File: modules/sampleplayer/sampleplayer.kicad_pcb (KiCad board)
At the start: 2 copper layers, 3 parts, among them J1 AudioJack2_SwitchT, U1 ESP32-DEVKIT-V1

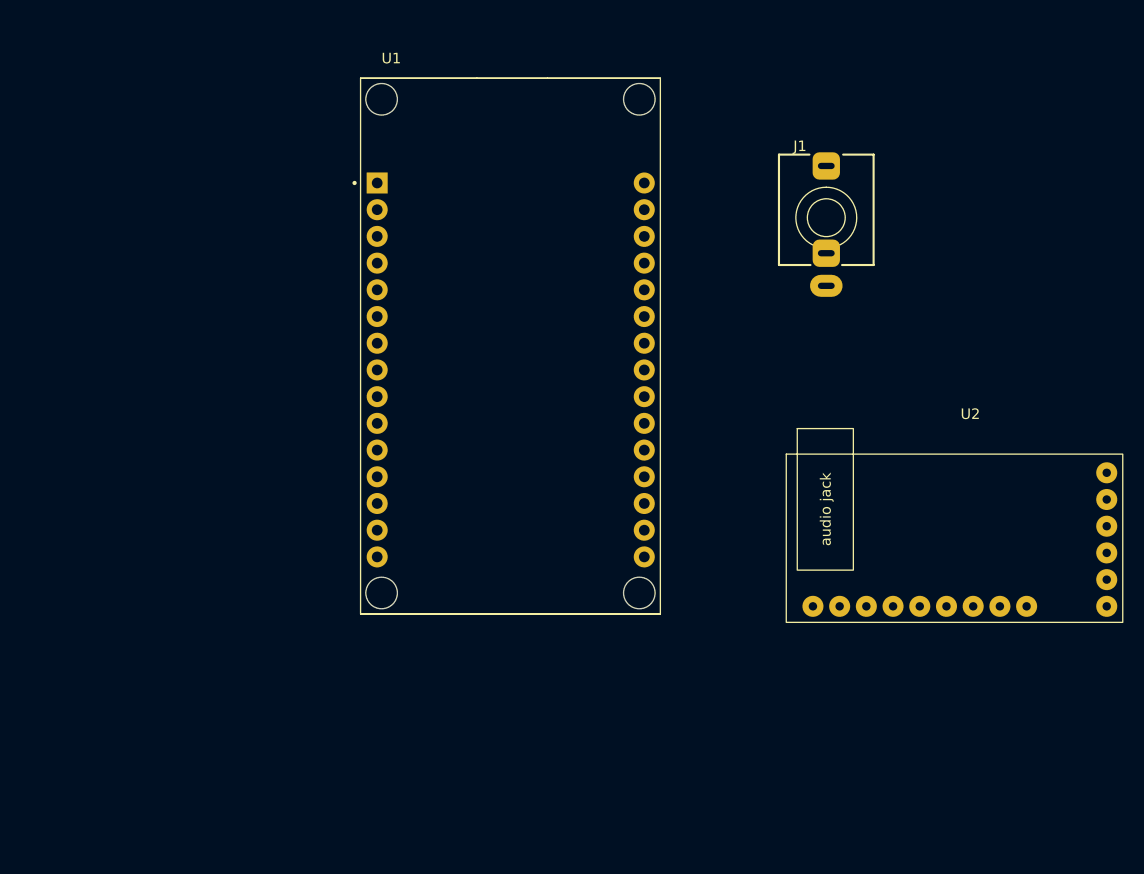
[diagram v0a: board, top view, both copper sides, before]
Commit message: sampleplayer update
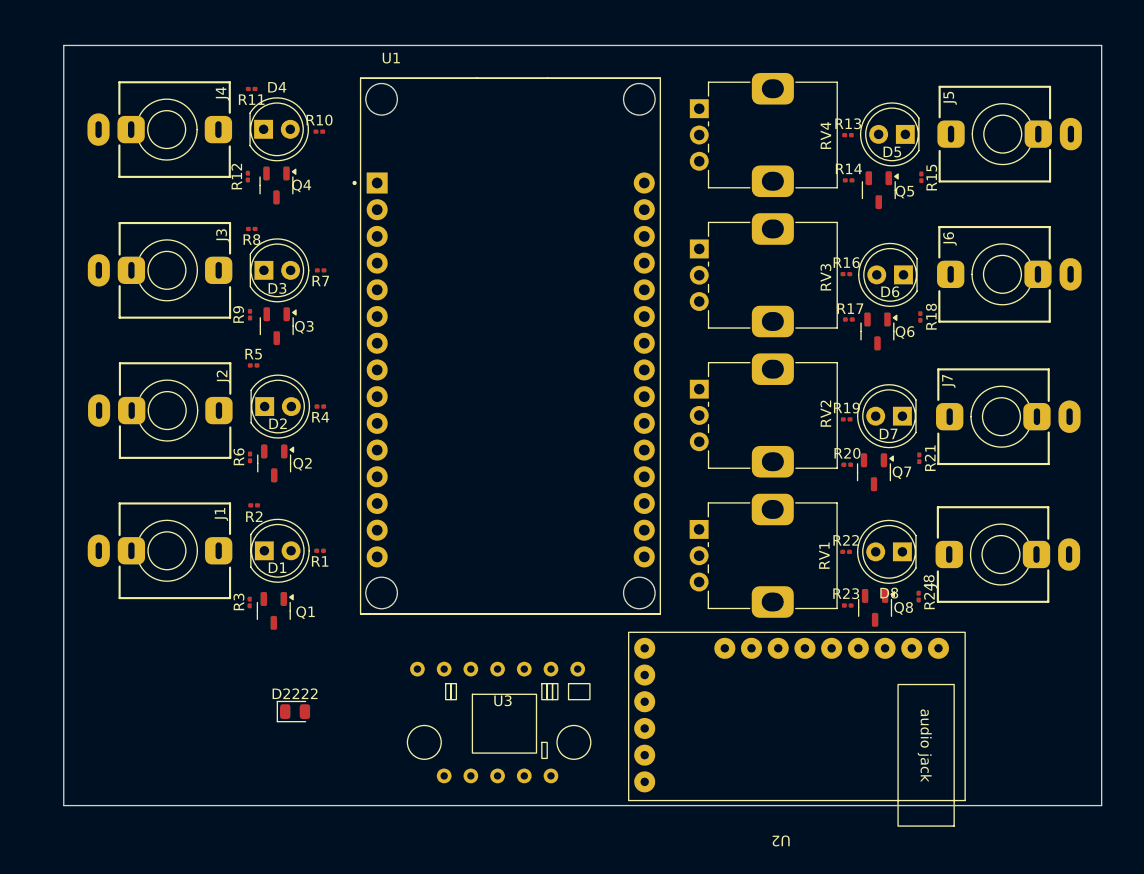
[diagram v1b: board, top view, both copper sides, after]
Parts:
- added D1: 5mm LED, LED_THT:LED_D5.0mm, F.Cu at (124.4, 123.0)
- added D2: 5mm LED, LED_THT:LED_D5.0mm, F.Cu at (124.4, 109.3)
- added D2222: KT-0805G, LED_SMD:LED_0805_2012Metric, F.Cu at (127.3, 138.3)
- added D3: 5mm LED, LED_THT:LED_D5.0mm, F.Cu at (124.3, 96.3)
- added D4: 5mm LED, LED_THT:LED_D5.0mm, F.Cu at (124.3, 82.9)
- added D5: 5mm LED, LED_THT:LED_D5.0mm, F.Cu at (185.3, 83.4)
- added D6: 5mm LED, LED_THT:LED_D5.0mm, F.Cu at (185.1, 96.7)
- added D7: 5mm LED, LED_THT:LED_D5.0mm, F.Cu at (185.0, 110.2)
- added D8: 5mm LED, LED_THT:LED_D5.0mm, F.Cu at (185.0, 123.1)
- added J1: trig1, AudioJacks:Jack_3.5mm_QingPu_WQP-PJ301M-12_Vertical, F.Cu at (115.1, 123.0)
- added J2: trig2, AudioJacks:Jack_3.5mm_QingPu_WQP-PJ301M-12_Vertical, F.Cu at (115.1, 109.7)
- added J3: trig3, AudioJacks:Jack_3.5mm_QingPu_WQP-PJ301M-12_Vertical, F.Cu at (115.1, 96.3)
- added J5: trig5, AudioJacks:Jack_3.5mm_QingPu_WQP-PJ301M-12_Vertical, F.Cu at (194.6, 83.4)
- added J6: trig6, AudioJacks:Jack_3.5mm_QingPu_WQP-PJ301M-12_Vertical, F.Cu at (194.6, 96.7)
- added J7: trig7, AudioJacks:Jack_3.5mm_QingPu_WQP-PJ301M-12_Vertical, F.Cu at (194.5, 110.2)
- added J8: trig8, AudioJacks:Jack_3.5mm_QingPu_WQP-PJ301M-12_Vertical, F.Cu at (194.4, 123.3)
- added Q1: SS8050, Package_TO_SOT_SMD:SOT-23-3, F.Cu at (125.3, 128.7)
- added Q2: SS8050, Package_TO_SOT_SMD:SOT-23-3, F.Cu at (125.3, 114.7)
- added Q3: SS8050, Package_TO_SOT_SMD:SOT-23-3, F.Cu at (125.5, 101.6)
- added Q4: SS8050, Package_TO_SOT_SMD:SOT-23-3, F.Cu at (125.5, 88.2)
- added Q5: SS8050, Package_TO_SOT_SMD:SOT-23-3, F.Cu at (182.8, 88.7)
- added Q6: SS8050, Package_TO_SOT_SMD:SOT-23-3, F.Cu at (182.7, 102.1)
- added Q7: SS8050, Package_TO_SOT_SMD:SOT-23-3, F.Cu at (182.3, 115.5)
- added Q8: SS8050, Package_TO_SOT_SMD:SOT-23-3, F.Cu at (182.4, 128.4)
- added R1: 56, Resistor_SMD:R_0201_0603Metric, F.Cu at (129.7, 123.0)
- added R10: 56, Resistor_SMD:R_0201_0603Metric, F.Cu at (129.6, 83.1)
- added R11: 330, Resistor_SMD:R_0201_0603Metric, F.Cu at (123.1, 79.1)
- added R12: 120K, Resistor_SMD:R_0201_0603Metric, F.Cu at (122.8, 87.4)
- added R13: 56, Resistor_SMD:R_0201_0603Metric, F.Cu at (179.9, 83.5)
- added R14: 330, Resistor_SMD:R_0201_0603Metric, F.Cu at (179.9, 87.8)
- added R15: 120K, Resistor_SMD:R_0201_0603Metric, F.Cu at (186.8, 87.5)
- added R16: 56, Resistor_SMD:R_0201_0603Metric, F.Cu at (179.7, 96.7)
- added R17: 330, Resistor_SMD:R_0201_0603Metric, F.Cu at (179.9, 101.0)
- added R18: 120K, Resistor_SMD:R_0201_0603Metric, F.Cu at (186.7, 100.7)
- added R19: 56, Resistor_SMD:R_0201_0603Metric, F.Cu at (179.7, 110.5)
- added R2: 330, Resistor_SMD:R_0201_0603Metric, F.Cu at (123.4, 118.7)
- added R20: 330, Resistor_SMD:R_0201_0603Metric, F.Cu at (179.8, 114.8)
- added R21: 120K, Resistor_SMD:R_0201_0603Metric, F.Cu at (186.6, 114.2)
- added R22: 56, Resistor_SMD:R_0201_0603Metric, F.Cu at (179.7, 123.1)
- added R23: 330, Resistor_SMD:R_0201_0603Metric, F.Cu at (179.8, 128.2)
- added R24: 120K, Resistor_SMD:R_0201_0603Metric, F.Cu at (186.6, 127.3)
- added R3: 120K, Resistor_SMD:R_0201_0603Metric, F.Cu at (123.0, 127.9)
- added R4: 56, Resistor_SMD:R_0201_0603Metric, F.Cu at (129.7, 109.3)
- added R5: 330, Resistor_SMD:R_0201_0603Metric, F.Cu at (123.3, 105.4)
- added R6: 120K, Resistor_SMD:R_0201_0603Metric, F.Cu at (123.0, 114.1)
- added R7: 56, Resistor_SMD:R_0201_0603Metric, F.Cu at (129.7, 96.3)
- added R8: 330, Resistor_SMD:R_0201_0603Metric, F.Cu at (123.2, 92.4)
- added R9: 120K, Resistor_SMD:R_0201_0603Metric, F.Cu at (123.0, 100.5)
- added RV1: R_Potentiometer, Potentiometer_THT:Potentiometer_Alps_RK09K_Single_Vertical, F.Cu at (165.7, 121.0)
- added RV2: R_Potentiometer, Potentiometer_THT:Potentiometer_Alps_RK09K_Single_Vertical, F.Cu at (165.7, 107.6)
- added RV3: R_Potentiometer, Potentiometer_THT:Potentiometer_Alps_RK09K_Single_Vertical, F.Cu at (165.7, 94.3)
- added RV4: R_Potentiometer, Potentiometer_THT:Potentiometer_Alps_RK09K_Single_Vertical, F.Cu at (165.7, 80.9)
- added U3: ~, breakoutboards:BMI160, F.Cu at (146.7, 139.2)
- J4: renamed from J1; value AudioJack2_SwitchT -> trig4
- U2: value ~ -> PCM5102
- moved J4 63.3 mm to (115.1, 82.9), turned to -90 degrees
- moved U2 23.4 mm to (174.0, 138.2), turned to 180 degrees
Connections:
- J4 pad S: unconnected-(J1-PadS) -> GND
- J4 pad T: unconnected-(J1-PadT) -> Net-(Q4-B)
- U1 pad 1: unconnected-(U1-3V3-Pad1) -> Net-(U1-3V3)
- U1 pad 11: unconnected-(U1-D21-Pad11) -> Net-(U1-D21)
- U1 pad 14: unconnected-(U1-D22-Pad14) -> Net-(U1-D22)
- U1 pad 17: unconnected-(U1-VP-Pad17) -> Net-(U1-VP)
- U1 pad 18: unconnected-(U1-VN-Pad18) -> Net-(U1-VN)
- U1 pad 19: unconnected-(U1-D34-Pad19) -> Net-(U1-D34)
- U1 pad 2: Net-(U1-GND-Pad2) -> GND
- U1 pad 20: unconnected-(U1-D35-Pad20) -> Net-(U1-D35)
- U1 pad 21: unconnected-(U1-D32-Pad21) -> Net-(U1-D32)
- U1 pad 22: unconnected-(U1-D33-Pad22) -> Net-(U1-D33)
- U1 pad 23: unconnected-(U1-D25-Pad23) -> Net-(U1-D25)
- U1 pad 24: unconnected-(U1-D26-Pad24) -> Net-(U1-D26)
- U1 pad 25: unconnected-(U1-D27-Pad25) -> Net-(U1-D27)
- U1 pad 26: unconnected-(U1-D14-Pad26) -> Net-(U1-D14)
- U1 pad 27: unconnected-(U1-D12-Pad27) -> Net-(U1-D12)
- U1 pad 28: unconnected-(U1-D13-Pad28) -> Net-(U1-D13)
- U1 pad 29: Net-(U1-GND-Pad2) -> GND
- U1 pad 3: unconnected-(U1-D15-Pad3) -> Net-(U1-D15)
- U1 pad 30: unconnected-(U1-VIN-Pad30) -> +5V
- U1 pad 4: unconnected-(U1-D2-Pad4) -> Net-(U1-D2)
- U1 pad 5: unconnected-(U1-D4-Pad5) -> Net-(U1-D4)
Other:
- board outline added: 98.7 x 72.3 mm

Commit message: sampleplayerupdate
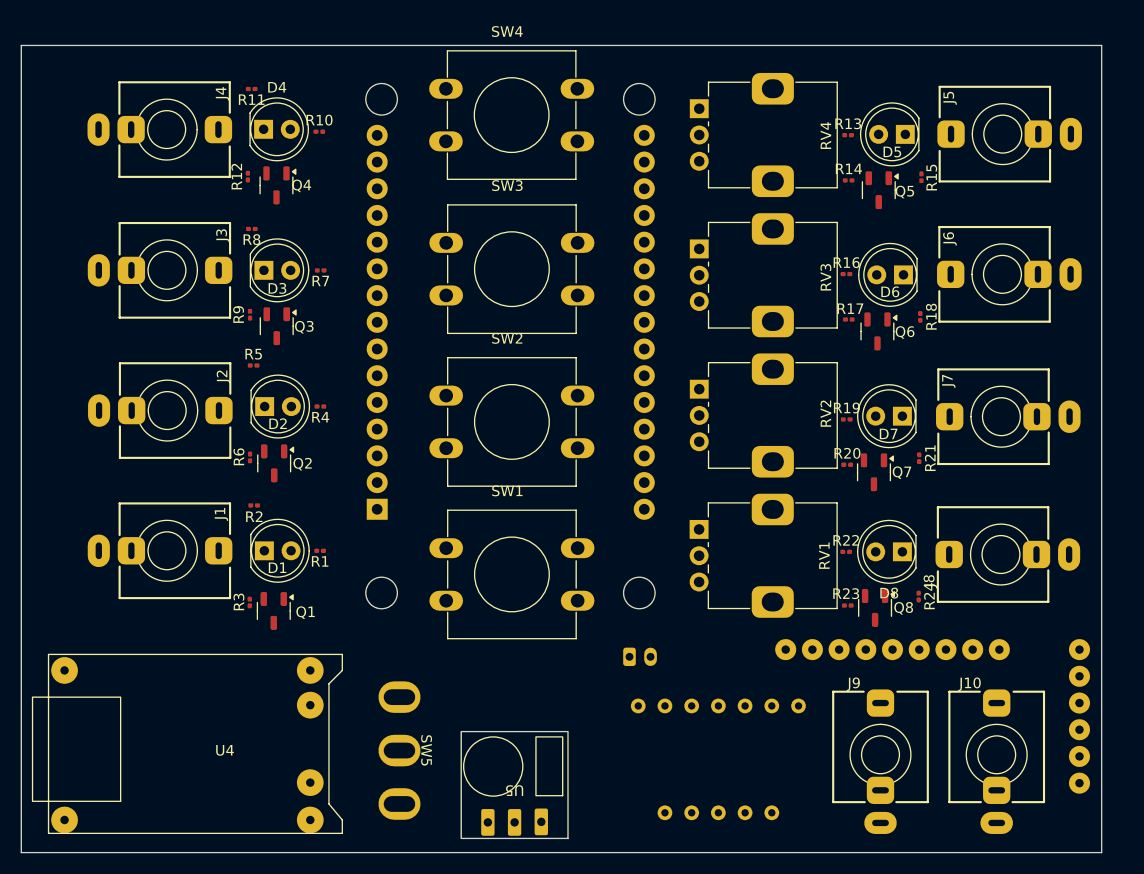
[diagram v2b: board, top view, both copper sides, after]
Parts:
- removed D2222: KT-0805G, LED_SMD:LED_0805_2012Metric
- added J10: audioL, AudioJacks:Jack_3.5mm_QingPu_WQP-PJ301M-12_Vertical, F.Cu at (194.0, 142.4)
- added J11: battery, Connector_JST:JST_PH_B2B-PH-K_1x02_P2.00mm_Vertical, B.Cu at (159.1, 133.1)
- added J9: audioR, AudioJacks:Jack_3.5mm_QingPu_WQP-PJ301M-12_Vertical, F.Cu at (183.0, 142.4)
- added SW1: SW_SPST, Button_Switch_THT:SW_PUSH-12mm, F.Cu at (141.7, 122.7)
- added SW2: SW_SPST, Button_Switch_THT:SW_PUSH-12mm, F.Cu at (141.7, 108.2)
- added SW3: SW_SPST, Button_Switch_THT:SW_PUSH-12mm, F.Cu at (141.7, 93.7)
- added SW4: SW_SPST, Button_Switch_THT:SW_PUSH-12mm, F.Cu at (141.6, 79.1)
- added SW5: SW_SPDT, breakoutboards:13x8mm_3pin, F.Cu at (138.5, 142.0)
- added U4: ~, breakoutboards:TP4056, F.Cu at (103.8, 149.9)
- added U5: ~, breakoutboards:DCDC5V, F.Cu at (148.2, 145.3)
- U1, U2, U3: moved to B.Cu
- moved U3 21.0 mm to (167.4, 142.7), turned to 180 degrees
- moved U2 14.5 mm to (188.5, 138.4), turned to 0 degrees
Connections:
- U1 pad 6: unconnected-(U1-RX2-D16-Pad6) -> Net-(SW1-A)
- U1 pad 7: unconnected-(U1-TX2-D17-Pad7) -> Net-(SW2-A)
- U1 pad 8: unconnected-(U1-D5-Pad8) -> Net-(SW3-A)
- U1 pad 9: unconnected-(U1-D18-Pad9) -> Net-(SW4-A)
- U2 pad 6: unconnected-(U2-AGND-Pad6) -> Net-(J9-PadS)
- U2 pad 7: unconnected-(U2-ROUT-Pad7) -> Net-(U2-ROUT)
- U2 pad 8: unconnected-(U2-AGND-Pad8) -> Net-(J10-PadS)
- U2 pad 9: unconnected-(U2-LRout-Pad9) -> Net-(U2-LRout)
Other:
- board size 98.7 x 72.3 mm -> 102.7 x 76.8 mm
